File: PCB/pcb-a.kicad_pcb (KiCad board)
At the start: 2 copper layers, 116.3 x 50.4 mm, 38 parts, among them Q1 BC337, Q2 BC337, Q3 BC337, Q4 BC337, SW1 config, U1 MCP23008-xP, U4 ATmega16L-8P

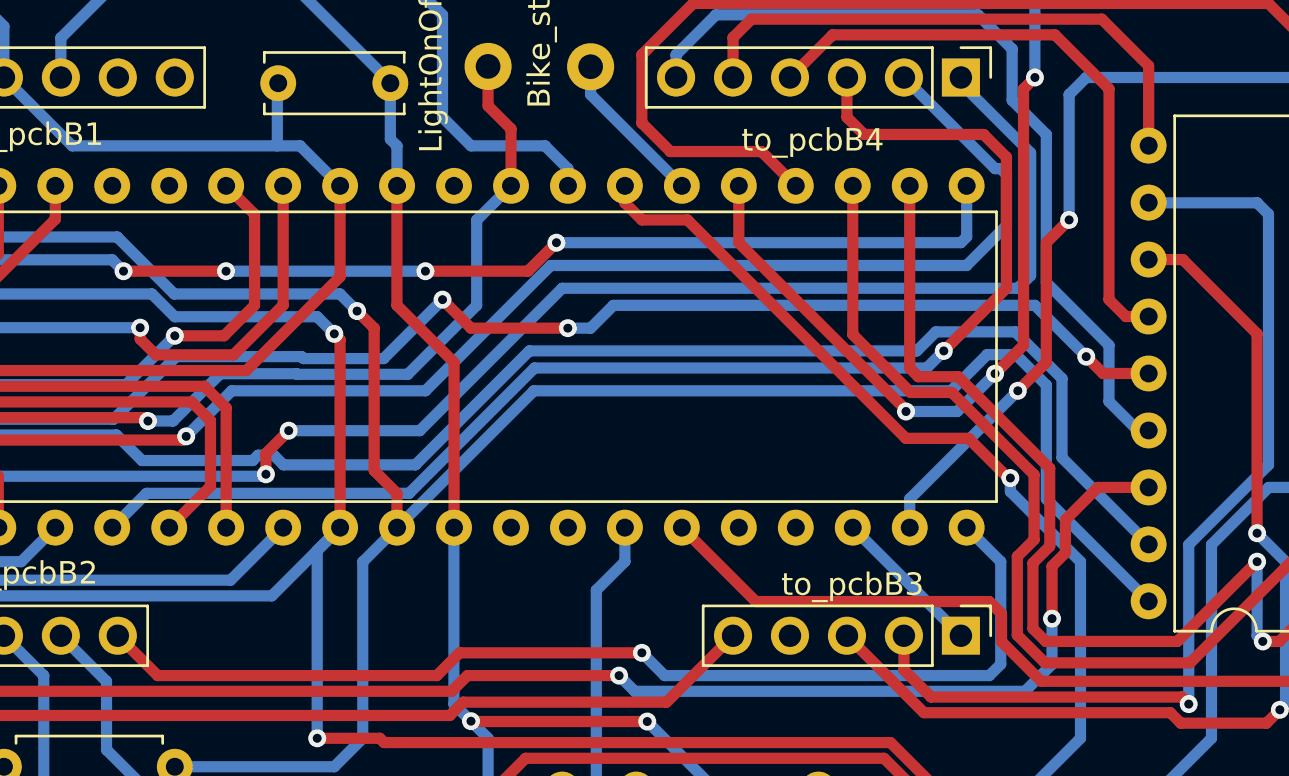
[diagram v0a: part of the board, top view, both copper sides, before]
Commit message: small errors and warnings fixed. Ready to be printed
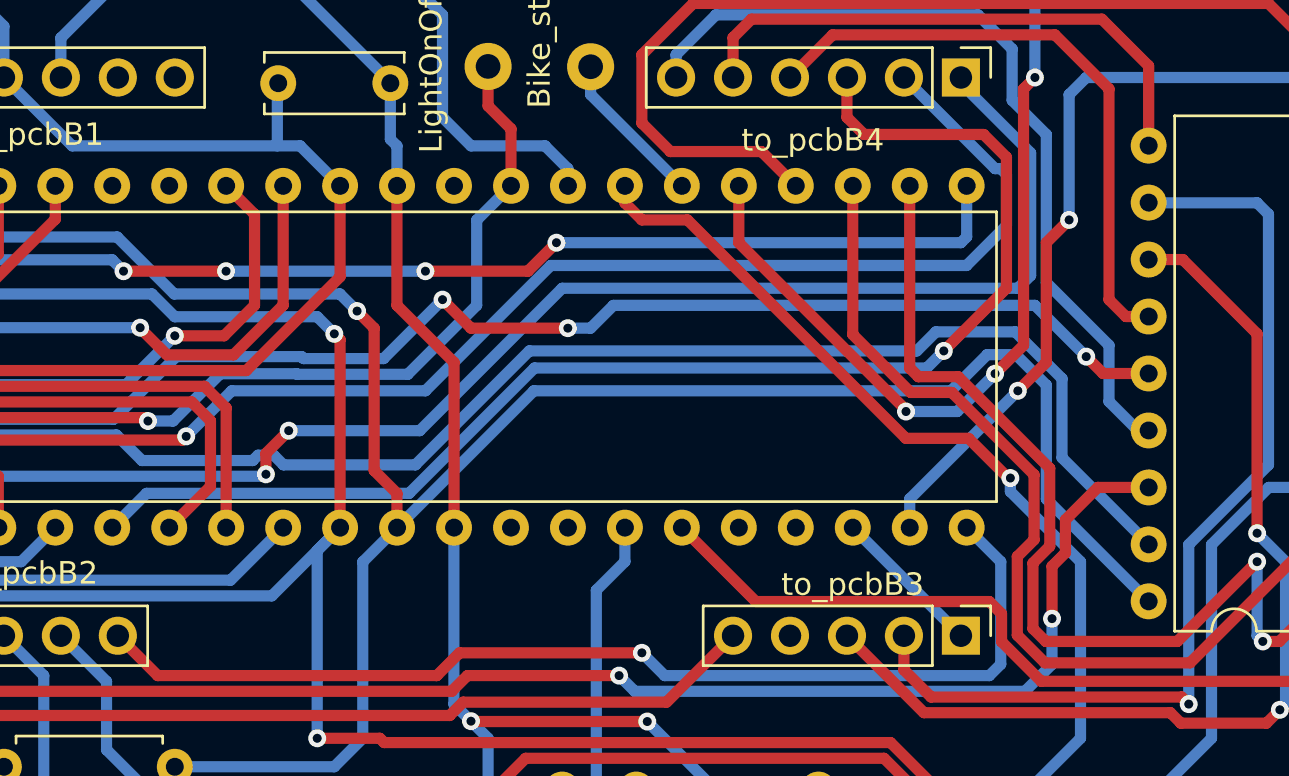
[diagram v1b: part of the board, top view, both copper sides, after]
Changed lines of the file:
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@@
   (segment (start 177.051 75.86505) (end 179.633262 78.447312) (width 0.5) (layer "F.Cu") (net 16))
   (segment (start 185.62 90.504) (end 192.094 90.504) (width 0.5) (layer "F.Cu") (net 16))
+  (segment (start 145.276 75.579582) (end 146.467918 76.7715) (width 0.5) (layer "F.Cu") (net 17))
+  (segment (start 149.4385 76.7715) (end 151.651 74.559) (width 0.5) (layer "F.Cu") (net 17))
+  (segment (start 145.276 75.56) (end 145.276 75.579582) (width 0.5) (layer "F.Cu") (net 17))
+  (segment (start 146.467918 76.7715) (end 149.4385 76.7715) (width 0.5) (layer "F.Cu") (net 17))
   (segment (start 151.651 74.559) (end 151.651 69.235) (width 0.5) (layer "F.Cu") (net 17))
-  (segment (start 145.276 76.068) (end 145.9795 76.7715) (width 0.5) (layer "F.Cu") (net 17))
-  (segment (start 145.276 75.56) (end 145.276 76.068) (width 0.5) (layer "F.Cu") (net 17))
-  (segment (start 145.9795 76.7715) (end 149.4385 76.7715) (width 0.5) (layer "F.Cu") (net 17))
-  (segment (start 149.4385 76.7715) (end 151.651 74.559) (width 0.5) (layer "F.Cu") (net 17))
   (via (at 145.276 75.56) (size 0.8) (drill 0.4) (layers "F.Cu" "B.Cu") (net 17))
-  (segment (start 145.276 75.56) (end 145.296 75.58) (width 0.5) (layer "B.Cu") (net 17))
   (segment (start 129.538 75.56) (end 145.276 75.56) (width 0.5) (layer "B.Cu") (net 17))
   (segment (start 149.0185 75.9215) (end 150.376 74.564) (width 0.5) (layer "F.Cu") (net 18))
@@
   (segment (start 144.6415 78.1) (end 129.538 78.1) (width 0.5) (layer "B.Cu") (net 18))
   (segment (start 181.872 89.296) (end 177.051 84.475) (width 0.5) (layer "B.Cu") (net 19))
-  (segment (start 182.126 89.042) (end 181.872 89.296) (width 0.5) (layer "B.Cu") (net 19))
   (segment (start 140.978 91.074) (end 139.2 89.296) (width 0.5) (layer "B.Cu") (net 20))
   (segment (start 139.1945 97.6835) (end 140.978 95.9) (width 0.5) (layer "B.Cu") (net 20))
@@
   (segment (start 171.712 62.626) (end 171.712 64.404) (width 0.5) (layer "F.Cu") (net 21))
   (segment (start 172.536 61.802) (end 171.712 62.626) (width 0.5) (layer "F.Cu") (net 21))
-  (segment (start 190 67.198) (end 190.244 67.442) (width 0.5) (layer "B.Cu") (net 21))
   (segment (start 180.224 92.728) (end 176.792 89.296) (width 0.5) (layer "F.Cu") (net 23))
   (segment (start 195.08 75.834) (end 191.768 72.522) (width 0.5) (layer "F.Cu") (net 23))
@@
   (segment (start 158.504 91.074) (end 146.058 91.074) (width 0.5) (layer "F.Cu") (net 66))
   (segment (start 167.648 90.058) (end 159.52 90.058) (width 0.5) (layer "F.Cu") (net 66))
-  (segment (start 182.126 84.48) (end 182.131 84.475) (width 0.5) (layer "F.Cu") (net 66))
   (via (at 167.648 90.058) (size 0.8) (drill 0.4) (layers "F.Cu" "B.Cu") (net 66))
   (segment (start 183.65 90.566) (end 183.65 85.994) (width 0.5) (layer "B.Cu") (net 66))
